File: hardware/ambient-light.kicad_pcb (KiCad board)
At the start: 2 copper layers, 25 x 15 mm, 16 parts, among them P1 CON-SENSOR, U1 M24C64, U2 LTR-329ALS, U3 DRILL, U4 DRILL, U5 DRILL, U6 DRILL

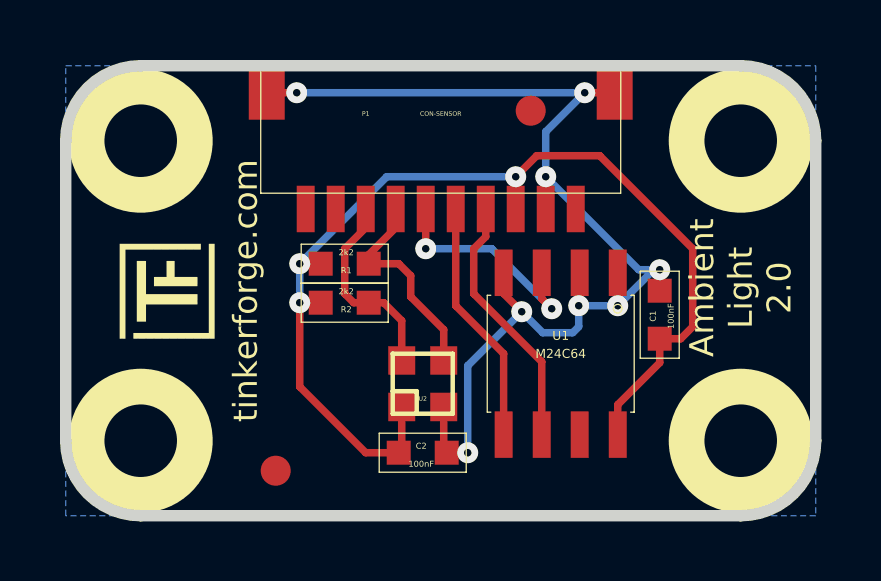
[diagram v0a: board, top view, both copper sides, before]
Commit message: Add 3d information (final)
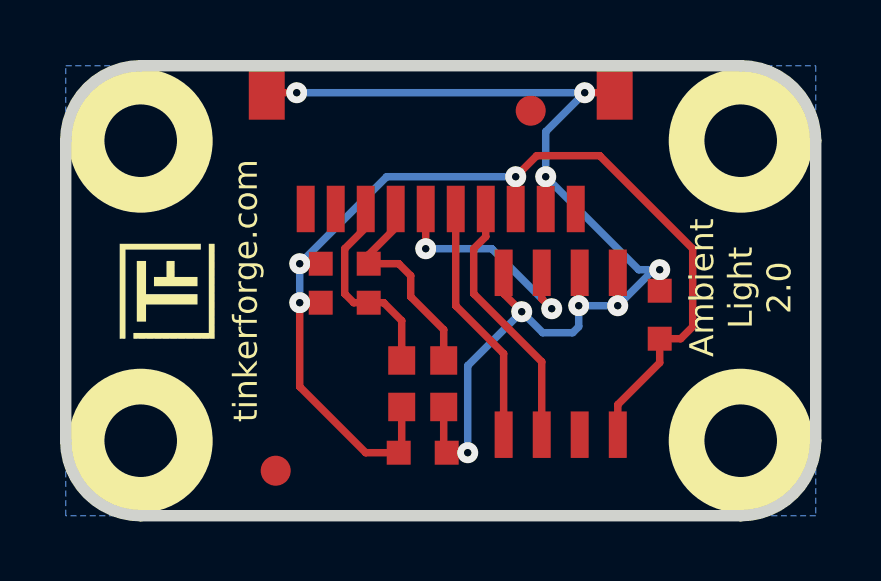
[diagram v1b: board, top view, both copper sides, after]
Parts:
- C1, C2: footprint kicad-libraries:0603 -> kicad-libraries:C0603
- R1, R2: footprint kicad-libraries:0603 -> kicad-libraries:R0603
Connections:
- P1 pad 1: (no net) -> Net-(P1-Pad1)
- P1 pad 10: (no net) -> Net-(P1-Pad10)
- P1 pad 9: (no net) -> Net-(P1-Pad9)
- U1 pad 7: (no net) -> Net-(U1-Pad7)
